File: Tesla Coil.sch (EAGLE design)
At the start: 1 part, among them IC1 NE555

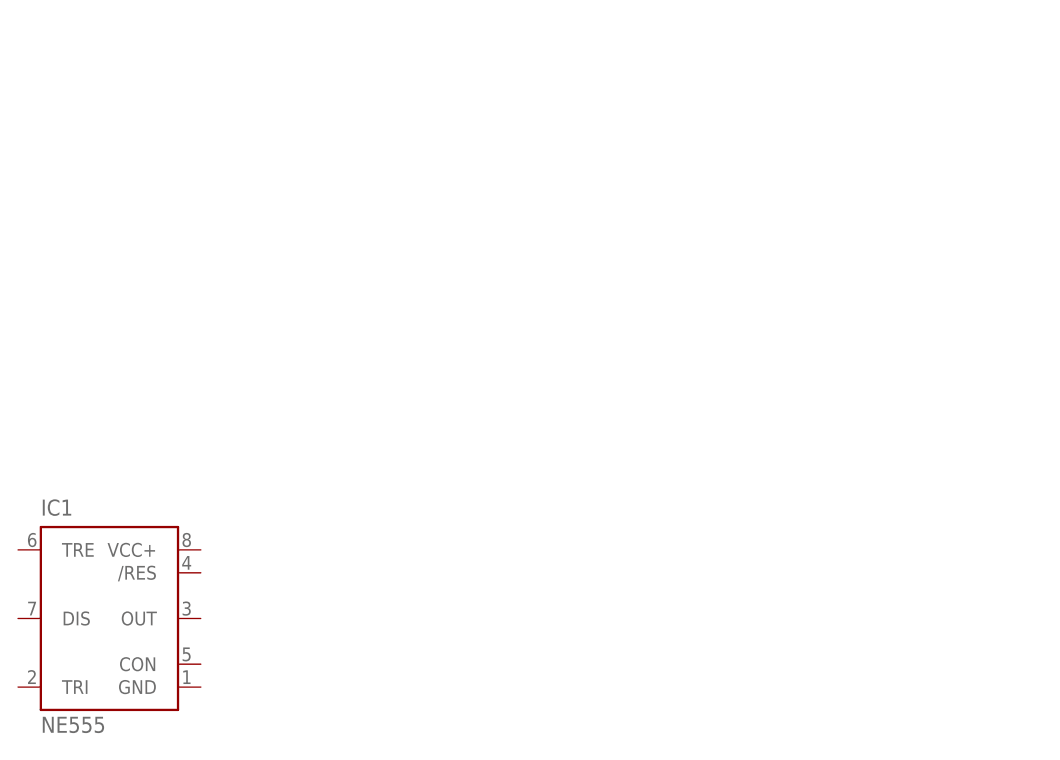
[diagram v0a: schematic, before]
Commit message: 2 lijntjes
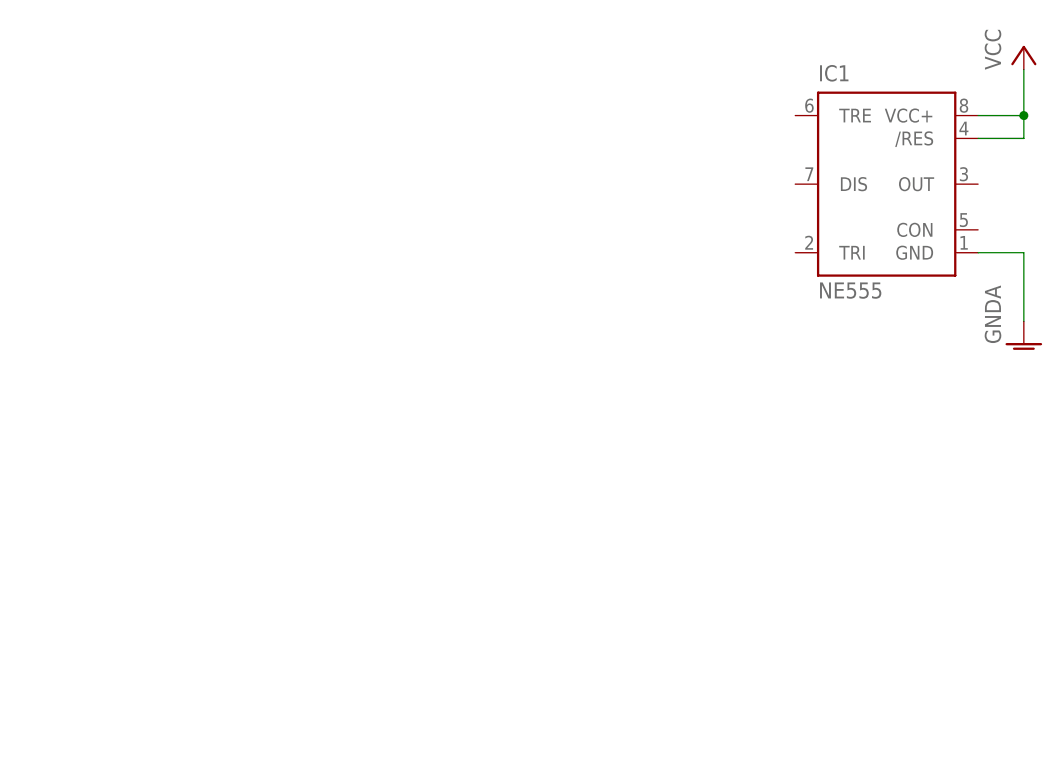
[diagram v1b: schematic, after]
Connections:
- new net GNDA: IC1.GND
- new net VCC: IC1./RES, IC1.VCC+
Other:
- moved on the sheet: IC1
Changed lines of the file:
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@@
 <part name="IC1" library="st-microelectronics" library_urn="urn:adsk.eagle:library:368" deviceset="NE555" device="" package3d_urn="urn:adsk.eagle:package:26829/1"/>
 <part name="FRAME1" library="frames" library_urn="urn:adsk.eagle:library:229" deviceset="DINA4_L" device=""/>
+<part name="GND1" library="supply1" library_urn="urn:adsk.eagle:library:371" deviceset="GNDA" device=""/>
+<part name="P+1" library="supply1" library_urn="urn:adsk.eagle:library:371" deviceset="VCC" device=""/>
 </parts>
 <sheets>
@@
 </plain>
 <instances>
-<instance part="IC1" gate="G$1" x="45.72" y="48.26" smashed="yes">
-<attribute name="NAME" x="38.1" y="59.69" size="1.778" layer="95"/>
-<attribute name="VALUE" x="38.1" y="35.56" size="1.778" layer="96"/>
+<instance part="IC1" gate="G$1" x="132.08" y="96.52" smashed="yes">
+<attribute name="NAME" x="124.46" y="107.95" size="1.778" layer="95"/>
+<attribute name="VALUE" x="124.46" y="83.82" size="1.778" layer="96"/>
 </instance>
 <instance part="FRAME1" gate="G$1" x="0" y="0" smashed="yes"/>
@@
 <attribute name="DRAWING_NAME" x="180.34" y="19.05" size="2.54" layer="94"/>
 </instance>
+<instance part="GND1" gate="1" x="147.32" y="78.74" smashed="yes">
+<attribute name="VALUE" x="144.78" y="78.74" size="1.778" layer="96" rot="R90"/>
+</instance>
+<instance part="P+1" gate="VCC" x="147.32" y="111.76" smashed="yes">
+<attribute name="VALUE" x="144.78" y="109.22" size="1.778" layer="96" rot="R90"/>
+</instance>
 </instances>
 <busses>
 </busses>
 <nets>
+<net name="GNDA" class="0">
+<segment>
+<pinref part="IC1" gate="G$1" pin="GND"/>
+<pinref part="GND1" gate="1" pin="GNDA"/>
+<wire x1="142.24" y1="88.9" x2="147.32" y2="88.9" width="0.1524" layer="91"/>
+<wire x1="147.32" y1="88.9" x2="147.32" y2="81.28" width="0.1524" layer="91"/>
+</segment>
+</net>
+<net name="VCC" class="0">
+<segment>
+<pinref part="IC1" gate="G$1" pin="VCC+"/>
+<pinref part="P+1" gate="VCC" pin="VCC"/>
+<wire x1="142.24" y1="104.14" x2="147.32" y2="104.14" width="0.1524" layer="91"/>
+<wire x1="147.32" y1="104.14" x2="147.32" y2="109.22" width="0.1524" layer="91"/>
+<pinref part="IC1" gate="G$1" pin="/RES"/>
+<wire x1="142.24" y1="101.6" x2="147.32" y2="101.6" width="0.1524" layer="91"/>
+<wire x1="147.32" y1="101.6" x2="147.32" y2="104.14" width="0.1524" layer="91"/>
+<junction x="147.32" y="104.14"/>
+</segment>
+</net>
 </nets>
 </sheet>
